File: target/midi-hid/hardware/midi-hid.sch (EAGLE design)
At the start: 128 parts, among them IC1 MEGA48/88/168-AU, SW1 EC12E_SW, SW2 EC12E_SW, SW3 EC12E_SW, SW4 EC12E_SW

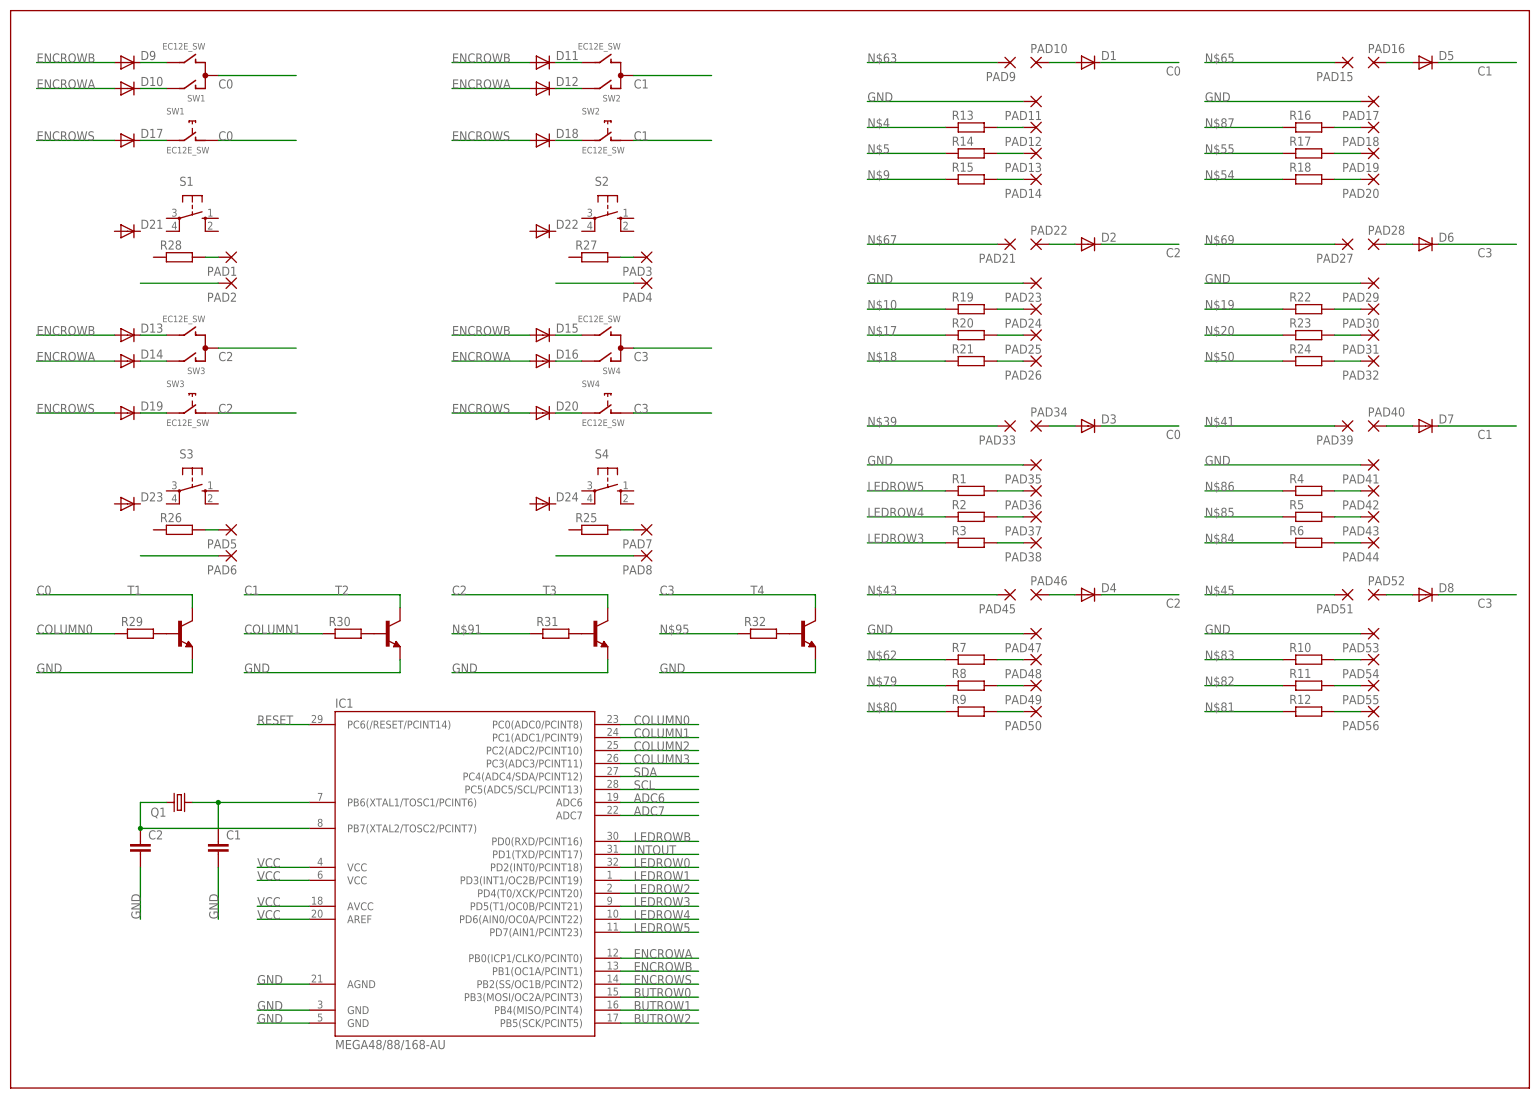
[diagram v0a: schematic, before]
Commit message: routing midi-hid
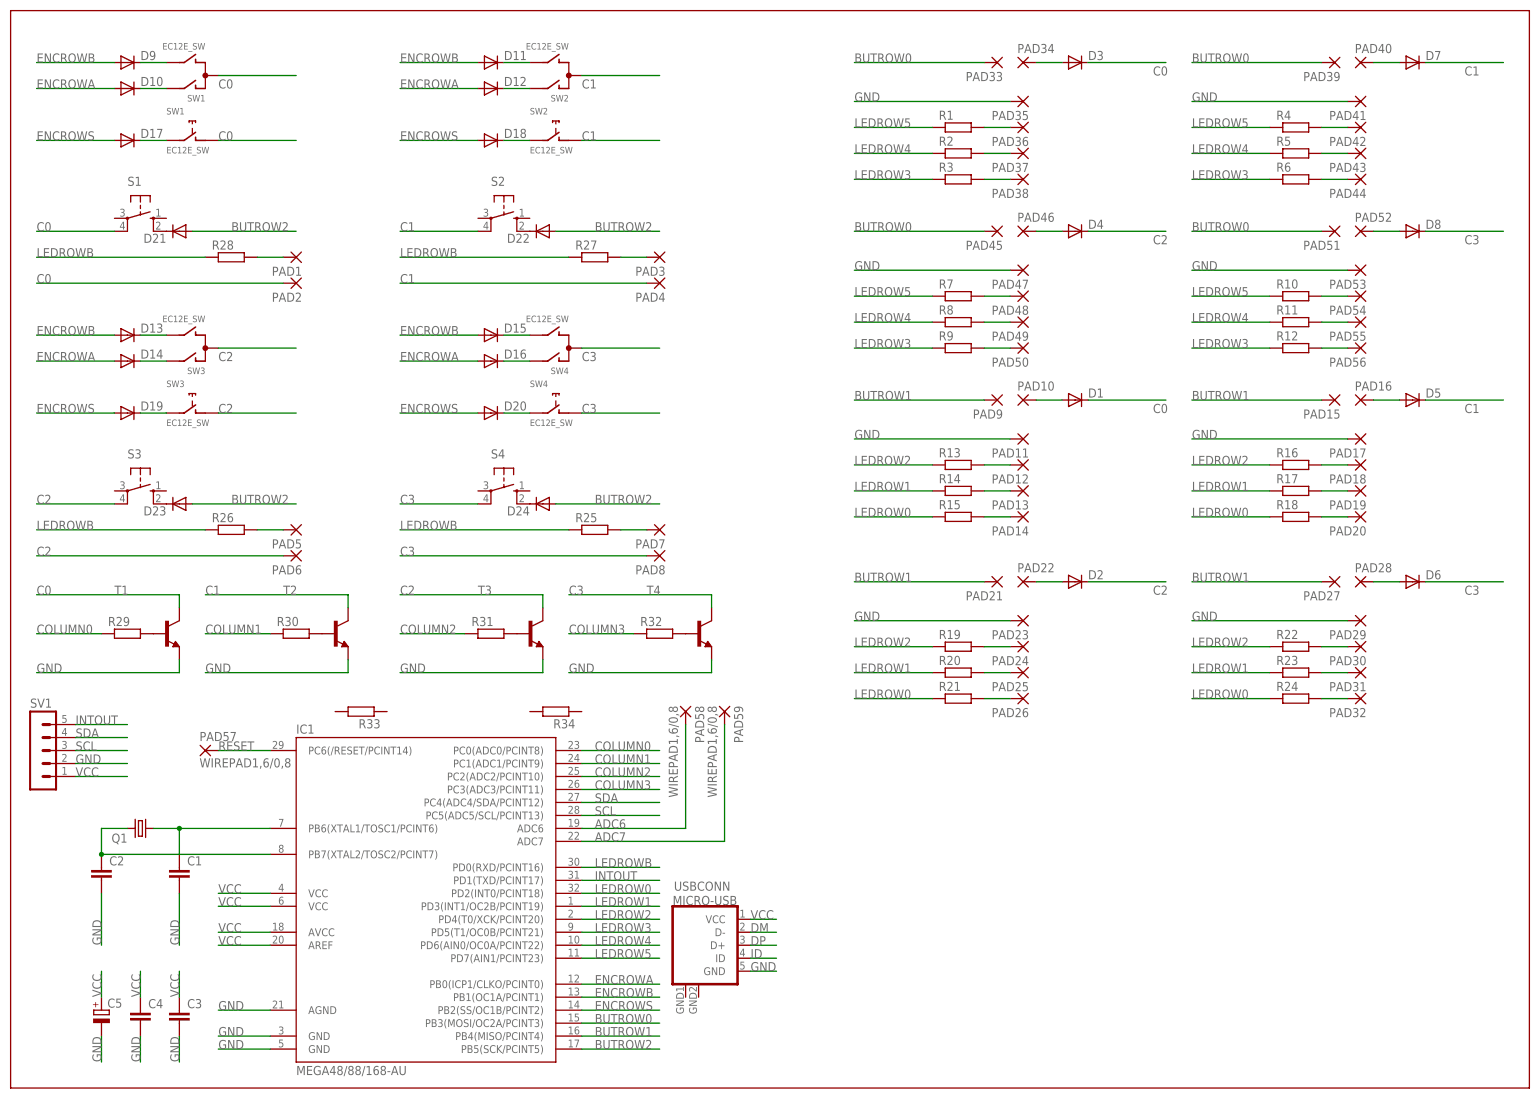
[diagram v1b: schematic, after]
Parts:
- added C3, C4: (no value), rcl:C-EUC0805
- added C5: (no value), rcl:CPOL-EUE2.5-6
- added PAD57, PAD58, PAD59: WIREPAD1,6/0,8, wirepad:WIREPAD1,6/0,8
- added R33, R34: (no value), rcl:R-EU_0207/10
- added SV1: (no value), con-lstb:MA05-1
- added USBCONN: MICRO-USB, microusb:MICRO-USB
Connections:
- removed net N$10: R19.1
- removed net N$17: R20.1
- removed net N$18: R21.1
- removed net N$19: R22.1
- removed net N$20: R23.1
- removed net N$39: PAD33.P
- removed net N$4: R13.1
- removed net N$41: PAD39.P
- removed net N$43: PAD45.P
- removed net N$45: PAD51.P
- removed net N$5: R14.1
- removed net N$50: R24.1
- removed net N$54: R18.1
- removed net N$55: R17.1
- removed net N$62: R7.1
- removed net N$63: PAD9.P
- removed net N$65: PAD15.P
- removed net N$67: PAD21.P
- removed net N$69: PAD27.P
- removed net N$71: PAD2.P
- removed net N$73: PAD4.P
- removed net N$75: PAD6.P
- removed net N$77: PAD8.P
- removed net N$79: R8.1
- removed net N$80: R9.1
- removed net N$81: R12.1
- removed net N$82: R11.1
- removed net N$83: R10.1
- removed net N$84: R6.1
- removed net N$85: R5.1
- removed net N$86: R4.1
- removed net N$87: R16.1
- removed net N$9: R15.1
- removed net N$95: R32.1
- new net DM: USBCONN.D-
- new net DP: USBCONN.D+
- new net ID: USBCONN.ID
- new net N$88: D22.C, S2.S1
- new net N$89: D21.C, S1.S1
- new net N$90: D23.C, S3.S1
- net ADC6: now also PAD58.P
- net ADC7: now also PAD59.P
- net BUTROW0: now also PAD33.P, PAD39.P, PAD45.P, PAD51.P
- net BUTROW1: now also PAD15.P, PAD21.P, PAD27.P, PAD9.P
- net BUTROW2: now also D21.A, D22.A, D23.A, D24.A
- net C0: now also PAD2.P, S1.P1
- net C1: now also PAD4.P, S2.P1
- net C2: now also PAD6.P, S3.P1
- net C3: now also PAD8.P, S4.P1
- net COLUMN2: now also R31.1
- net COLUMN3: now also R32.1
- net GND: now also C3.2, C4.2, C5.-, SV1.2, USBCONN.GND
- net INTOUT: now also SV1.5
- net LEDROW0: now also R15.1, R18.1, R21.1, R24.1
- net LEDROW1: now also R14.1, R17.1, R20.1, R23.1
- net LEDROW2: now also R13.1, R16.1, R19.1, R22.1
- net LEDROW3: now also R12.1, R6.1, R9.1
- net LEDROW4: now also R11.1, R5.1, R8.1
- net LEDROW5: now also R10.1, R4.1, R7.1
- net LEDROWB: now also R25.1, R26.1, R27.1, R28.1
- net N$91: now also D24.C, S4.S1; no longer R31.1
- net RESET: now also PAD57.P
- net SCL: now also SV1.3
- net SDA: now also SV1.4
- net VCC: now also C3.1, C4.1, C5.+, SV1.1, USBCONN.VCC
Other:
- moved on the sheet: C1, C2, D1, D11, D12, D15, D16, D18, D2, D20, D21, D22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
